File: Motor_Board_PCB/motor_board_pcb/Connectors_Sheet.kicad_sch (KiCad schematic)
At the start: 10 parts, among them J11 CSP-USC16-TR, J7 Conn_01x03, J8 Conn_01x02

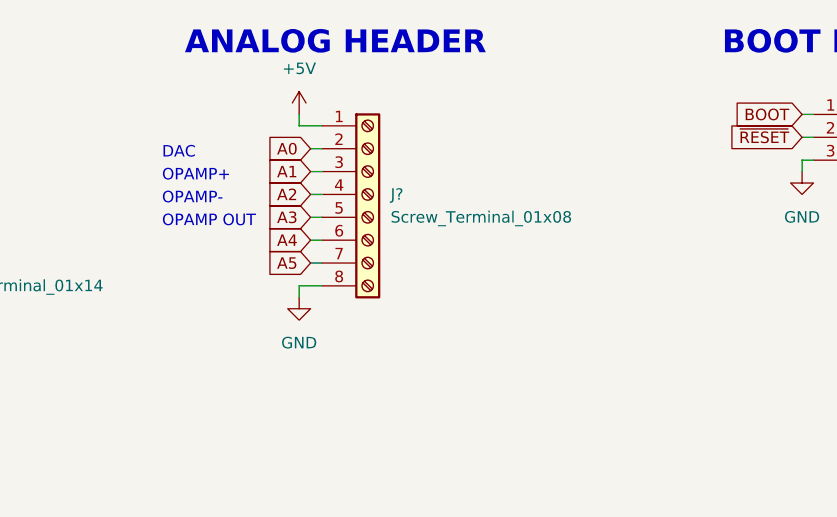
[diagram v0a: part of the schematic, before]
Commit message: Schematic changes before sending to kim
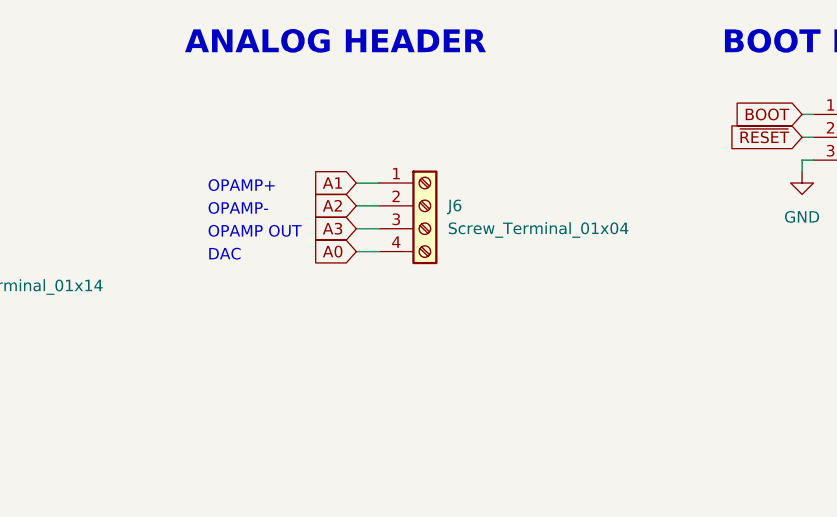
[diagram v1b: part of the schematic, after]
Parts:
- removed J?: Screw_Terminal_01x08, Connector_PinHeader_2.54mm:PinHeader_1x08_P2.54mm_Vertical, symbol Connector:Screw_Terminal_01x08
- added J6: Screw_Terminal_01x04, Connector_PinHeader_2.54mm:PinHeader_1x04_P2.54mm_Vertical, symbol Connector:Screw_Terminal_01x04
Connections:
- net A0: now also J6.4
- net A1: now also J6.1
- net A2: now also J6.2
- net A3: now also J6.3
